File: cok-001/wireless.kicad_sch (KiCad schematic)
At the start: 12 parts, among them J3701 Conn_01x33_MountingPin

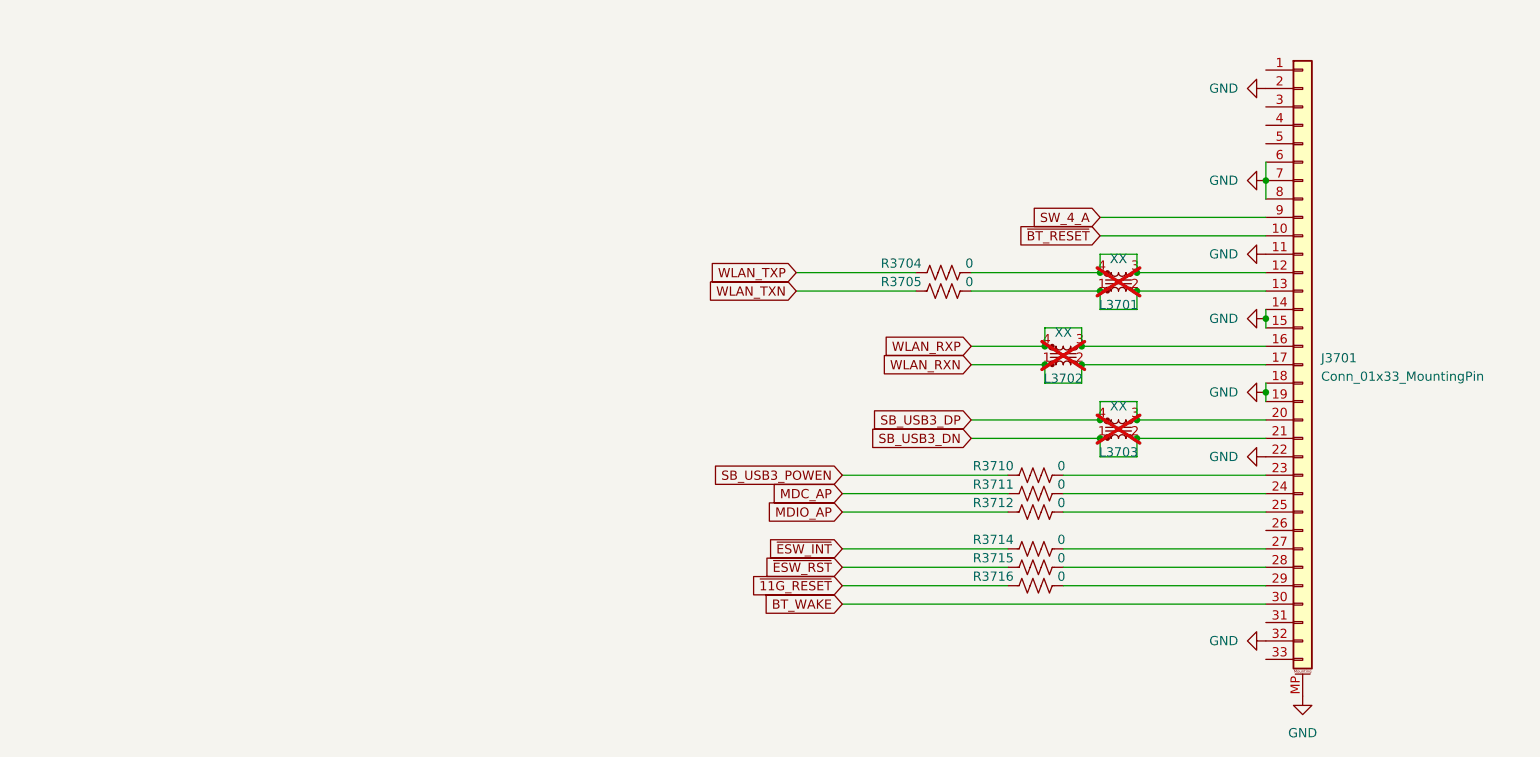
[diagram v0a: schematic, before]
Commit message: tx led
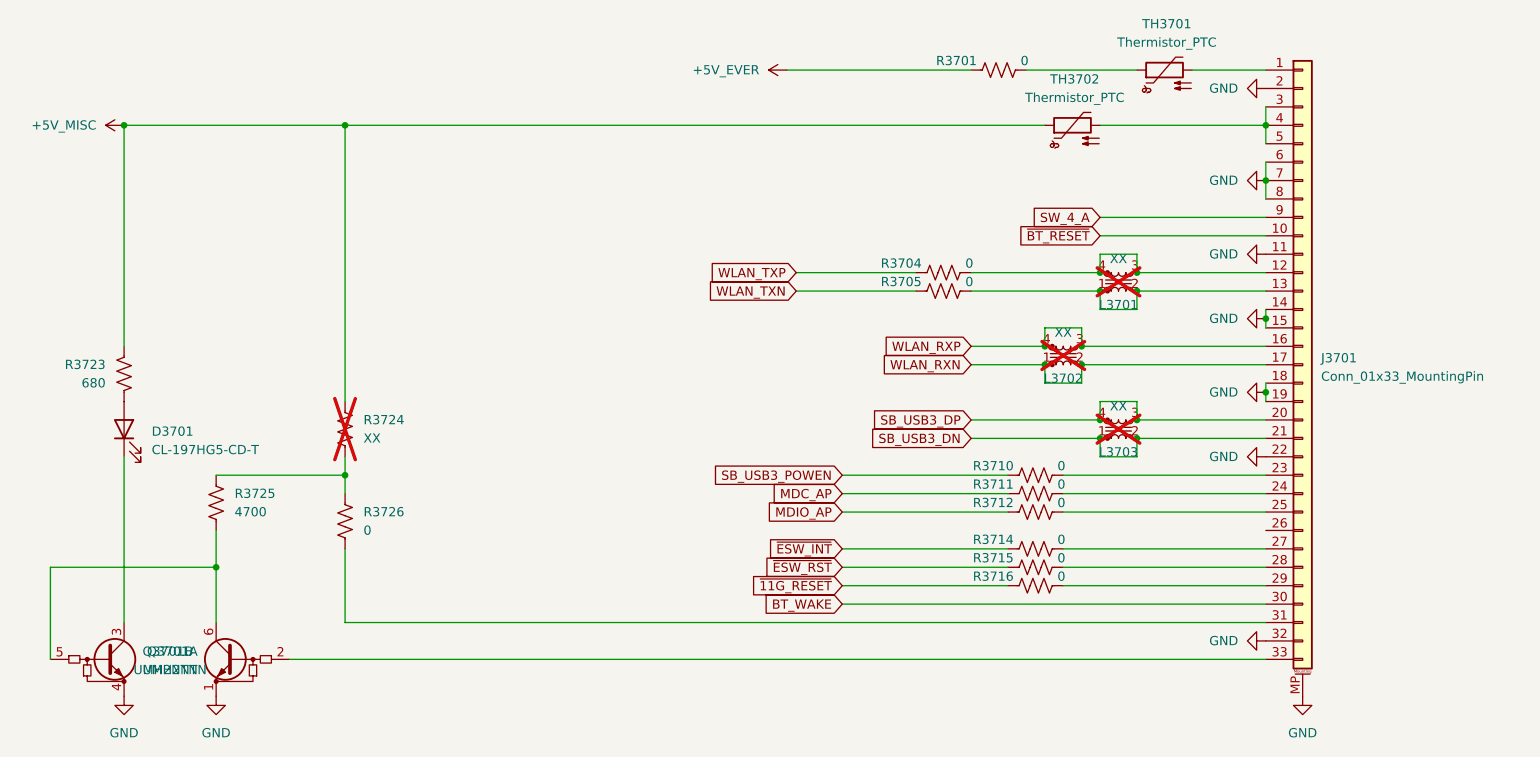
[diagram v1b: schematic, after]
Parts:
- added D3701: CL-197HG5-CD-T, Diode_SMD:D_0603_1608Metric, symbol Device:LED
- added Q3701: UMH2NTN, Package_TO_SOT_SMD:SOT-363_SC-70-6, symbol Transistor_BJT:MUN5213DW1
- added R3701: 0, Resistor_SMD:R_0805_2012Metric, symbol Device:R_US
- added R3723: 680, Resistor_SMD:R_0402_1005Metric, symbol Device:R_US
- added R3724: XX, Resistor_SMD:R_0402_1005Metric, symbol Device:R_US
- added R3725: 4700, Resistor_SMD:R_0402_1005Metric, symbol Device:R_US
- added R3726: 0, Resistor_SMD:R_0402_1005Metric, symbol Device:R_US
- added TH3701, TH3702: Thermistor_PTC, symbol Device:Thermistor_PTC
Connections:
- net GND: now also Q3701.1 (E1), Q3701.4 (E2)
- net at J3701.1 (Pin_1): now also TH3701.2
- net at J3701.3 (Pin_3): now also J3701.4 (Pin_4), J3701.5 (Pin_5), TH3702.2
- net at J3701.31 (Pin_31): now also R3726.2
- net at J3701.33 (Pin_33): now also Q3701.2 (B1)
- new net: R3701.2, TH3701.1
- new net: Q3701.5 (B2), Q3701.6 (C1), R3725.2
- new net: R3724.2, R3725.1, R3726.1
- new net: D3701.1 (K), Q3701.3 (C2)
- new net: D3701.2 (A), R3723.2
- new net +5V_EVER: R3701.1
- new net +5V_MISC: R3723.1, R3724.1, TH3702.1
